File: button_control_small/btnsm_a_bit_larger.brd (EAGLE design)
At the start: 40.9 x 40.9 mm, 77 parts, among them IC1 LP298XS, IC2 MEGA8-AI, IC3 FM24-SG, J1 AVR_SPI_PROG_3X2NS, J2 OUT-, J3 OUT+, Q1 310mA/60V/1.6Ω, Q2 4.3A/20V/54mΩ, Q3 4.3A/20V/54mΩ, Q4 310mA/60V/1.6Ω, Q5 4.3A/20V/54mΩ, Q6 3.6864MHz, T1 BC848, T2 BC848, T3 BC848, T4 BC848, T5 BC848, U1 ACS711ELCTR-25AB-T, U2 HC_05, U3 DS18B20

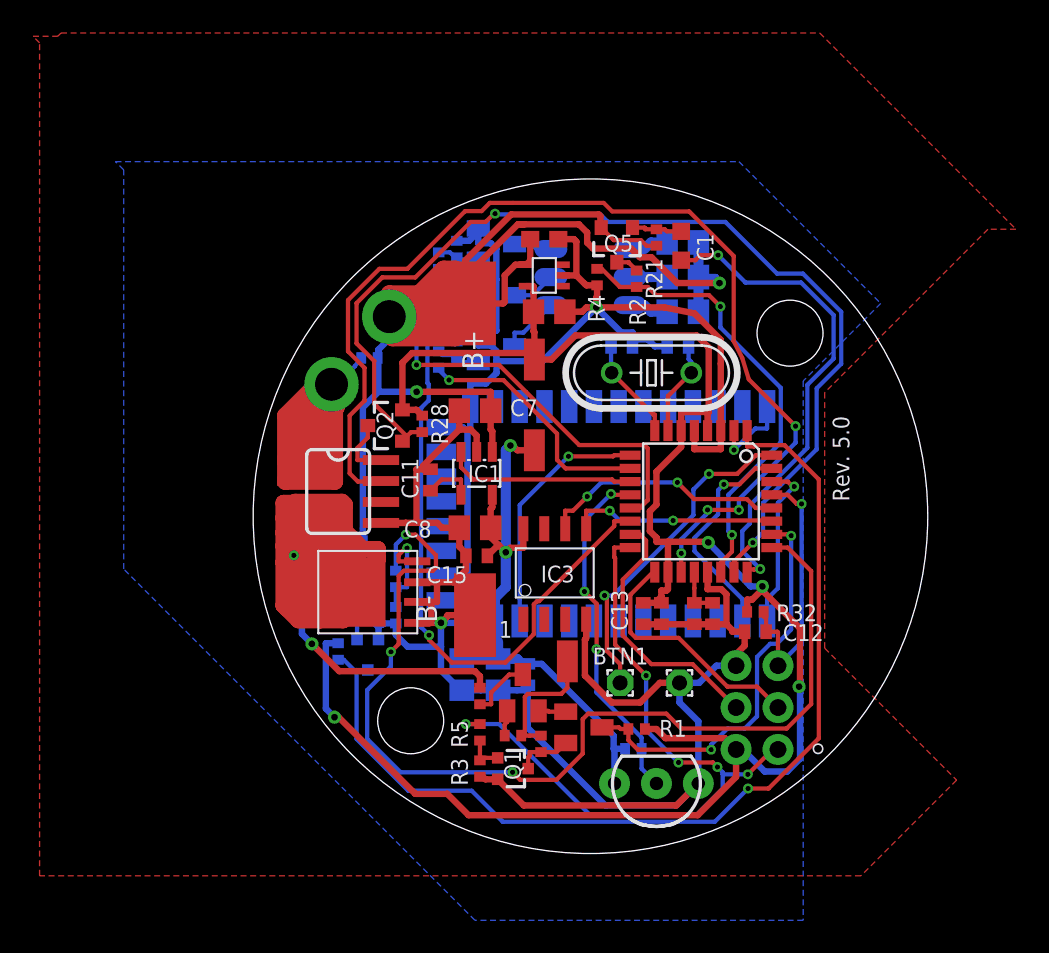
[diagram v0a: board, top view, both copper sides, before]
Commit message: Bump to 5.8
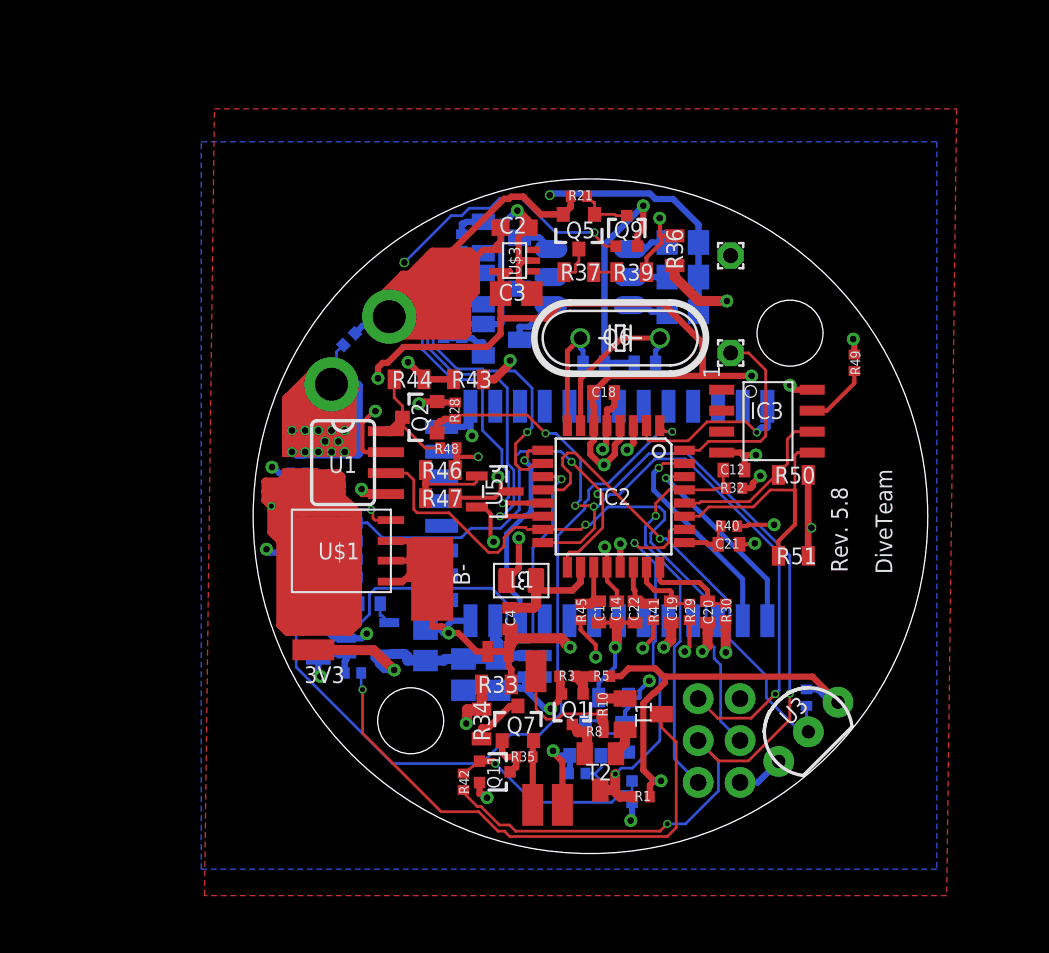
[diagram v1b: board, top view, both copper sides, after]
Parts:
- removed 3V3_CONST: 3V_SW, wirepad:SMD1,27-2,54
- removed 3V3_SWITCHED: 3V3, wirepad:SMD1,27-2,54
- removed C13: 10n, resistor:C0402
- removed C5: 100n, resistor:C0402
- added 3V3: 3V3, wirepad:SMD1,27-2,54
- added 4.2: 4.2, wirepad:SMD1,27-2,54
- added 8.4: 8.4, wirepad:SMD1,27-2,54
- added C18: 100n, resistor:C0402
- added C19, C20, C21, C22: 10n, resistor:C0402
- added L1: 10UH-225MA, Seeed-Inductor:L0806
- added Q10, Q11, Q9: 310mA/60V/1.6Ω, SparkFun-DiscreteSemi:SOT323
- added Q7, Q8: 4.3A/20V/54mΩ, SparkFun-DiscreteSemi:SOT23-3
- added R29, R30, R35, R38, R40, R41, R45, R49: 100k, rcl:R0402
- added R33, R36, R43, R44: 100k 1%, SparkFun-Resistors:0805
- added R34: 200k 1%, SparkFun-Resistors:0805
- added R37: 120k 1%, SparkFun-Resistors:0805
- added R39: 270k 1%, SparkFun-Resistors:0805
- added R42: 1k, rcl:R0402
- added R46: 1.2k 1%, SparkFun-Resistors:0805
- added R47, R50, R51: 6.2k 1%, SparkFun-Resistors:0805
- added R48: 200, rcl:R0402
- added SUPPLY7: 2PT_GND_TIE, SparkFun-PowerSymbols:2PT_GND_TIE
- added U5: TL431BQDBZR, TL431BQDBZR:SOT95P237X112-3N
- C1: value 100n -> 10n; device resistor:C0603K -> resistor:C0402
- R2: value 282k -> 100k 1%; device rcl:R0402 -> SparkFun-Resistors:0805
- R4: value 100k -> 200k 1%; device rcl:R0402 -> SparkFun-Resistors:0805
- moved R2 27.8 mm to (22.1, 6.60), flipped to the bottom
- moved BTN2 26.1 mm to (28.5, 35.8)
- moved R4 25.5 mm to (21.4, 9.00), flipped to the bottom, turned to 180 degrees
- moved C1 22.8 mm to (20.5, 14.2), turned to 270 degrees
- moved BTN1 21.1 mm to (28.5, 29.9)
- moved C7 16.8 mm to (3.50, 12.6), flipped to the bottom, turned to 90 degrees
- moved IC3 16.7 mm to (30.7, 26.4), turned to 270 degrees
- moved IC1 12.0 mm to (6.50, 12.6), flipped to the bottom, turned to 90 degrees
- moved R31 10.9 mm to (33.1, 9.00), turned to 90 degrees
- moved C12 9.89 mm to (28.7, 22.8), turned to 0 degrees
- moved U3 9.73 mm to (33.2, 6.93), turned to 45 degrees
- moved C4 9.20 mm to (15.1, 13.8)
- moved C11 8.36 mm to (6.60, 14.7), flipped to the bottom, turned to 0 degrees
- moved R5 8.14 mm to (20.7, 10.3), turned to 0 degrees
- moved C15 7.85 mm to (17.2, 10.9), flipped to the bottom, turned to 270 degrees
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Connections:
- removed net MOSI: IC2.15, J1.4
- removed net PC0: IC2.23, Q2.1, R28.1
- removed net PC1: C1.1, IC2.24
- removed net PC2: IC2.25, R19.2
- removed net PWR_MEASURE_VCC: Q2.3, U1.8
- removed net SCK: IC2.17, J1.3
- new net ADC0: R29.2, R36.2, R39.2
- new net ADC1: R30.2, R33.2, R34.1
- new net ADC2: R2.1, R4.2, R40.2
- new net AGND: C1.2, C14.2, C19.2, C20.2, C21.2, C22.2, C4.2, R33.1, R36.1, R4.1, R43.1, R47.1, SUPPLY7.P$2, U5.3
- new net AVCC: C4.1, IC2.18, L1.2
- new net N$10: 8.4.1, Q7.2, R35.2
- new net N$12: 4.2.1, Q8.2, R38.2
- new net N$14: Q2.3, R44.2, R48.2, U1.8
- new net N$19: Q10.1, Q11.1, Q9.1, R42.1
- new net N$26: IC3.7, R49.1
- new net N$3: Q11.3, Q7.1, R35.1
- new net N$5: Q7.3, R34.2
- new net N$6: Q10.3, Q8.1, R38.1
- new net N$7: Q8.3, R2.2
- new net N$8: R37.1, R39.1
- new net PB3/MOSI: IC2.15, J1.4, U1.6
- new net PB5/SCK: IC2.17, J1.3, R19.2, R42.2
- new net REF: R46.1, R47.2, U5.1
- new net _A0: C19.1, IC2.23, R29.1
- new net _A1: C20.1, IC2.24, R30.1
- new net _A2: C21.1, IC2.25, R40.1
- new net _A6: C1.1, IC2.19, R45.1
- new net _A7: C22.1, IC2.22, R41.1
- net ADC6: now also R43.2, R44.1, R45.2; no longer IC2.19, U1.7
- net ADC7: now also R41.2, U1.7; no longer IC2.22, R2.2, R4.1
- net AREF: now also R46.2, R48.1, U5.2; no longer C5.2
- net GND: now also C18.2, Q10.2, Q11.2, Q9.2, R49.2, SUPPLY7.P$1; no longer C13.2, C14.2, C4.2, C5.1, R4.2
- net N$11: now also Q9.3; no longer C1.2
- net N$23: now also R37.2; no longer R2.1
- net PB4/MISO: now also Q2.1, R28.1; no longer R5.2
- net SCL: now also R50.1
- net SDA: now also R51.1
- net VCC: now also 3V3.1, R1.2, R5.2, R50.2, R51.2; no longer 3V3_SWITCHED.1
- net VDD: now also C18.1, L1.1; no longer 3V3_CONST.1, C13.1, C4.1, IC2.18, R1.2
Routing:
- net GND_OUT: track 39.9 -> 232.5 mm, vias 0 -> 12
- net AGND: track 0.00 -> 82.9 mm, vias 0 -> 8
- net PB5/SCK: track 0.00 -> 80.4 mm, vias 0 -> 4
- net N$19: track 0.00 -> 65.6 mm, vias 0 -> 3
- net PC0: track 63.4 -> 0.00 mm, vias 2 -> 0
- net VCC: track 37.3 -> 100.4 mm, vias 2 -> 4
- net PC2: track 61.5 -> 0.00 mm, vias 3 -> 0
- net GND_OUT_MEASURE: track 76.7 -> 127.9 mm
- net GND: track 185.8 -> 231.6 mm, vias 2 -> 14
- net ADC0: track 0.00 -> 40.6 mm, vias 0 -> 2
- net PB3/MOSI: track 0.00 -> 38.0 mm, vias 0 -> 1
- net +12V: track 122.8 -> 159.8 mm
- net ADC6: track 65.1 -> 29.7 mm, vias 4 -> 2
- net PC1: track 30.0 -> 0.00 mm, vias 2 -> 0
- net WTR_MEASURE_PULLUP: track 3.76 -> 32.8 mm, vias 0 -> 1
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- added copper zone on layer 15, net AGND
- added copper zone on layer 15, net GND
- added copper zone on layer 2, net GND
- added copper zone on layer 15, net N$15
- added copper zone on layer 2, net N$16
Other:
- board text added: "DiveTeam"
- board text added: "Rev. 5.8"
- board text removed: "B+"
- board text removed: "Rev. 5.0"
